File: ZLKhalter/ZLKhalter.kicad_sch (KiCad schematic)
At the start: 7 parts, among them J1 Conn_02x04_Counter_Clockwise, J2 Conn_01x04_Pin, J3 Conn_02x04_Counter_Clockwise, J4 Conn_02x03_Odd_Even, J6 Conn_02x03_Top_Bottom, J7 Conn_02x03_Top_Bottom

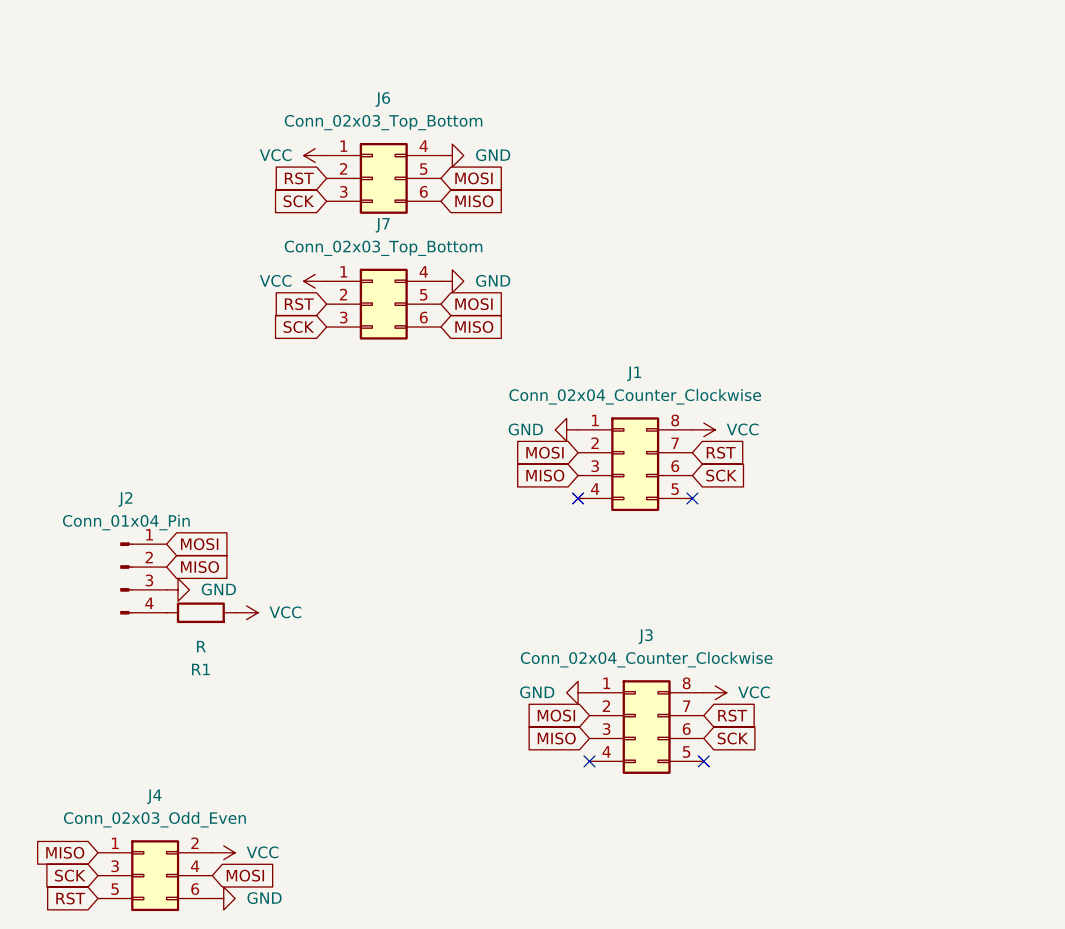
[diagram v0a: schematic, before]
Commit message: 12v zlk
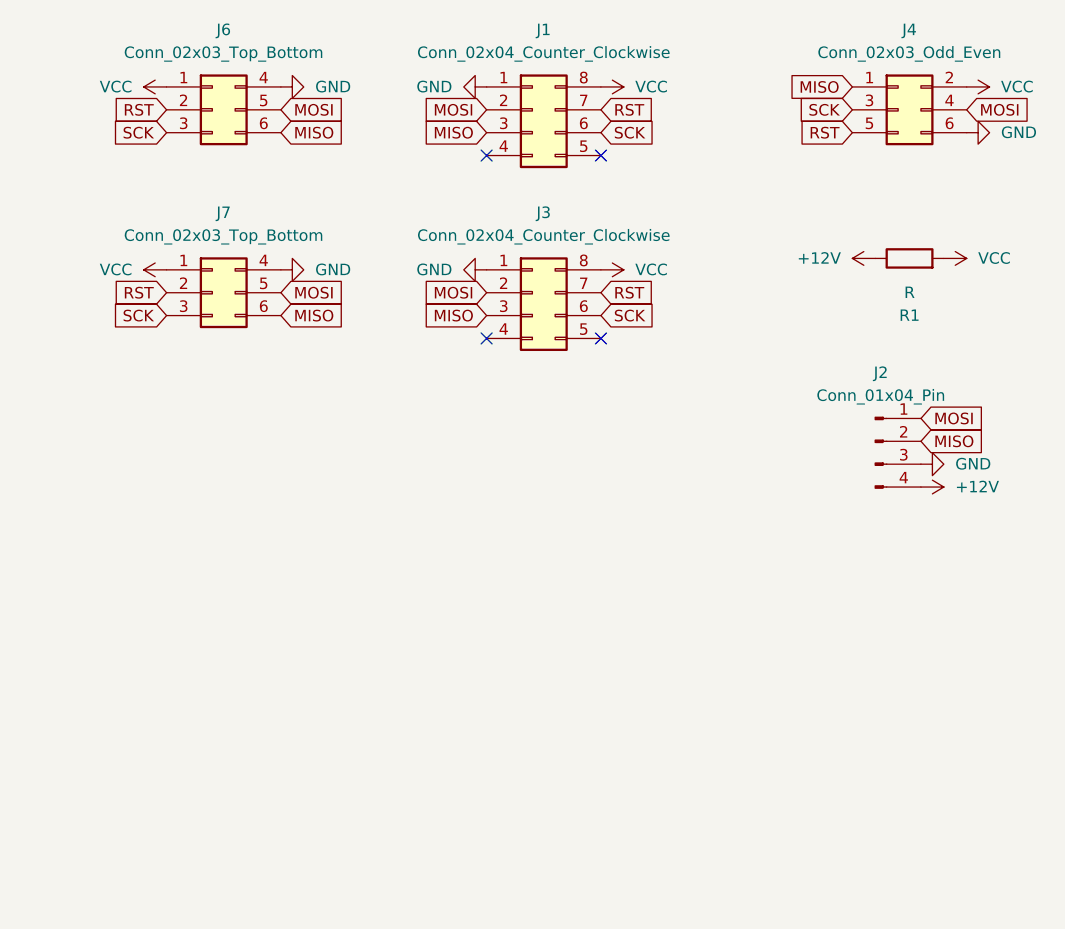
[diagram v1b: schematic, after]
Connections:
- net +12V: now reaches J2.4 (Pin_4), R1.1
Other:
- moved on the sheet: J1, J2, J3, J4, J6, J7, R1
